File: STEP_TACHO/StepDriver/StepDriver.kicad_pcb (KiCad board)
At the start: 2 copper layers, 31.8 x 35.6 mm, 15 parts, among them J1 STEP-MOTOR, J2 H:0.5V/L:0.125V, J3 M1, J4 M2, J5 DCY, J6 I/F, J7 POWER, U1 TB6608FNG

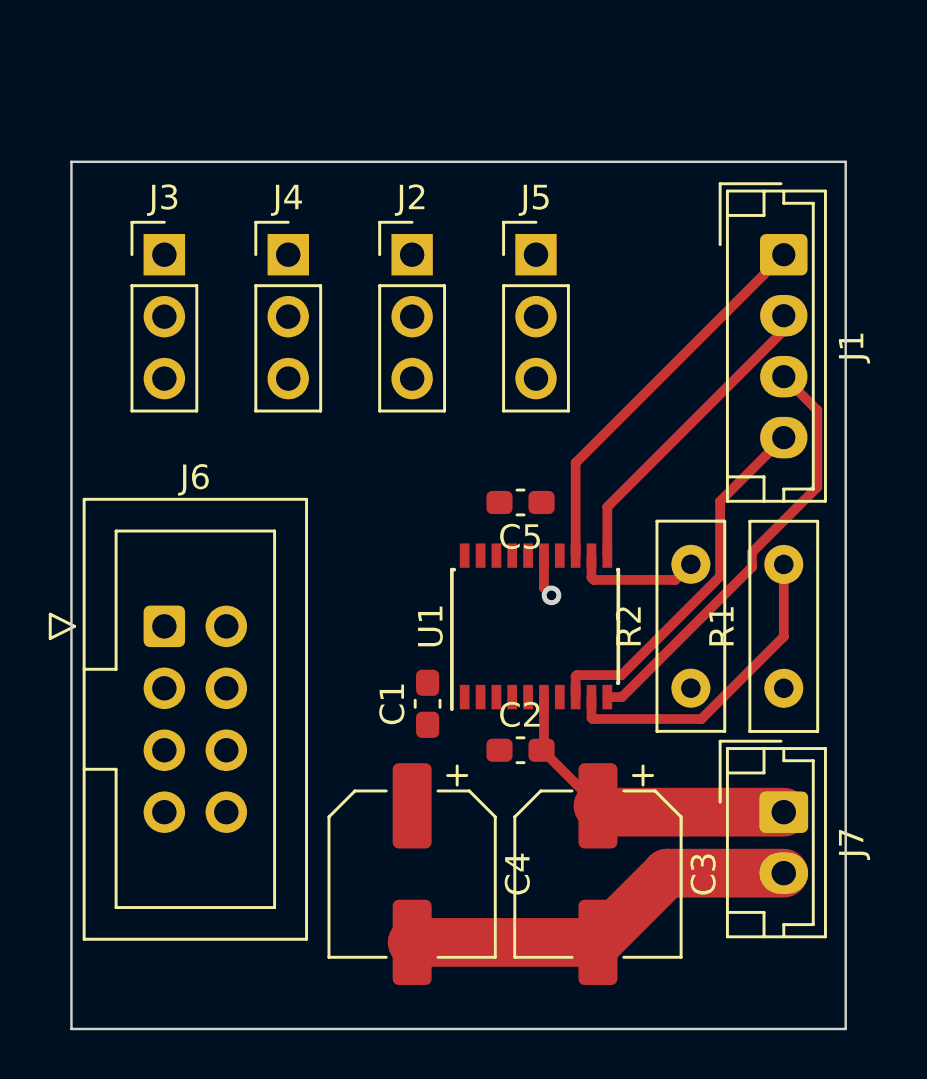
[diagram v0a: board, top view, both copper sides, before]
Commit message: Update: cleanup
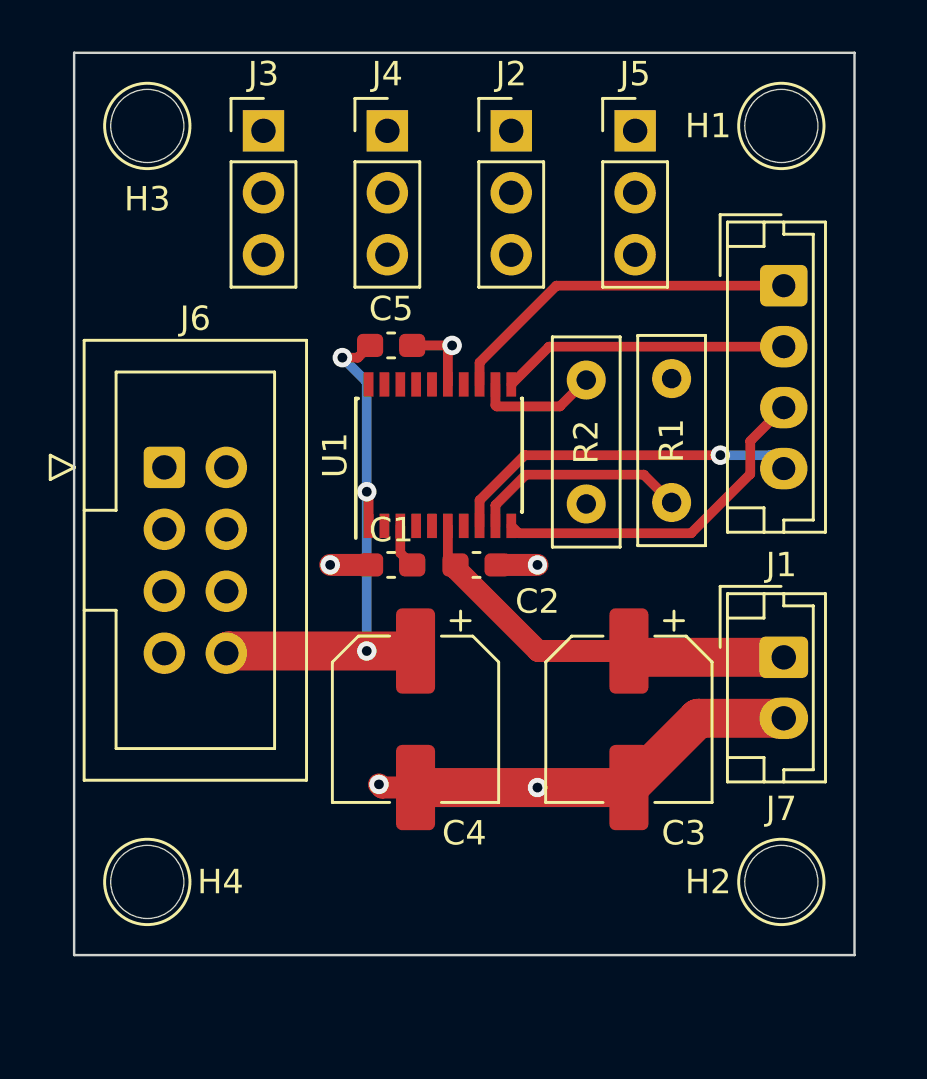
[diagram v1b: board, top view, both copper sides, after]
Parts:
- added H1: 3mm, KiCAD_lib:Hole3mm, F.Cu at (165.0, 76.0)
- added H2: 3mm, KiCAD_lib:Hole3mm, F.Cu at (165.0, 107.0)
- added H3: 3mm, KiCAD_lib:Hole3mm, F.Cu at (139.0, 76.0)
- added H4: 3mm, KiCAD_lib:Hole3mm, F.Cu at (139.0, 107.0)
- moved R1 13.5 mm to (160.5, 86.4), turned to -90 degrees
- moved R2 8.69 mm to (157.0, 91.5)
- moved C5 8.34 mm to (149.0, 85.0)
- moved U1 8.05 mm to (151.0, 89.5)
- moved C2 7.81 mm to (152.5, 94.0), turned to 180 degrees
- moved J6 6.52 mm to (139.7, 90.0)
- moved J3 6.51 mm to (143.8, 76.2)
- moved J2 6.51 mm to (153.9, 76.2)
- moved J4 6.51 mm to (148.8, 76.2)
- moved J5 6.51 mm to (159.0, 76.2)
- moved C3 6.48 mm to (158.8, 100.3)
- moved C4 6.35 mm to (150.0, 100.3)
- moved J7 6.35 mm to (165.1, 97.8)
- moved C1 5.89 mm to (149.0, 94.0), turned to 0 degrees
- moved J1 1.27 mm to (165.1, 82.5)
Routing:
- net VCC: track 0.00 -> 23.0 mm, vias 0 -> 3
- net GND: track 18.2 -> 24.4 mm, vias 1 -> 5
- net Net-(U1-RFB): track 13.1 -> 9.06 mm
- net VDD: track 13.1 -> 16.8 mm
- net Net-(J1-Pin_3): track 17.6 -> 14.2 mm
- net Net-(U1-OSC): track 0.00 -> 1.80 mm
- net Net-(J1-Pin_1): track 15.9 -> 14.7 mm
- net Net-(J1-Pin_2): track 12.8 -> 11.8 mm
- net Net-(J1-Pin_4): track 15.2 -> 14.5 mm, vias 0 -> 1
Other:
- board size 31.8 x 35.6 mm -> 32 x 37 mm
